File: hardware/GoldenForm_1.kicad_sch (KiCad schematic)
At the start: 37 parts, among them IC1 UVLO, J1 SD_Socket, J2 USB_C_Receptacle_USB2.0_14P, J3 Conn_01x04_Pin, M3 MountingHole x 4, SW1 BOOT, SW2 RESET, U1 Buck_Boost, U2 BNO055, U4 ESP32-S3-WROOM-1

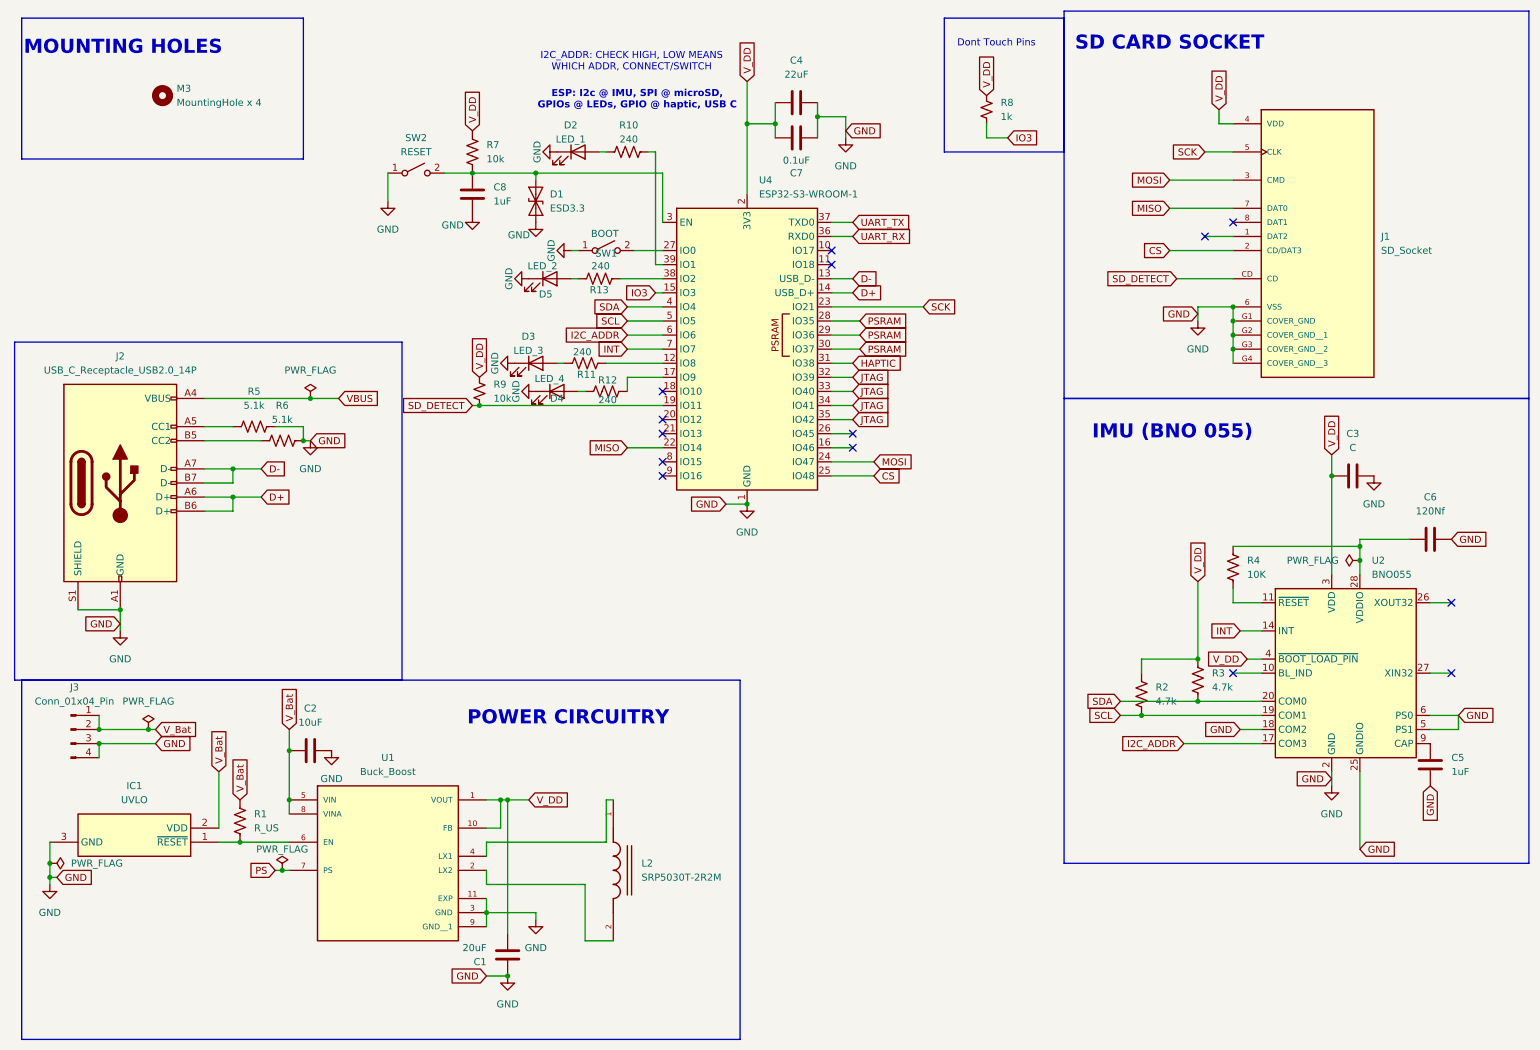
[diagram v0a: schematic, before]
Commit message: some updates to footprints, USBC, buck boost, switch
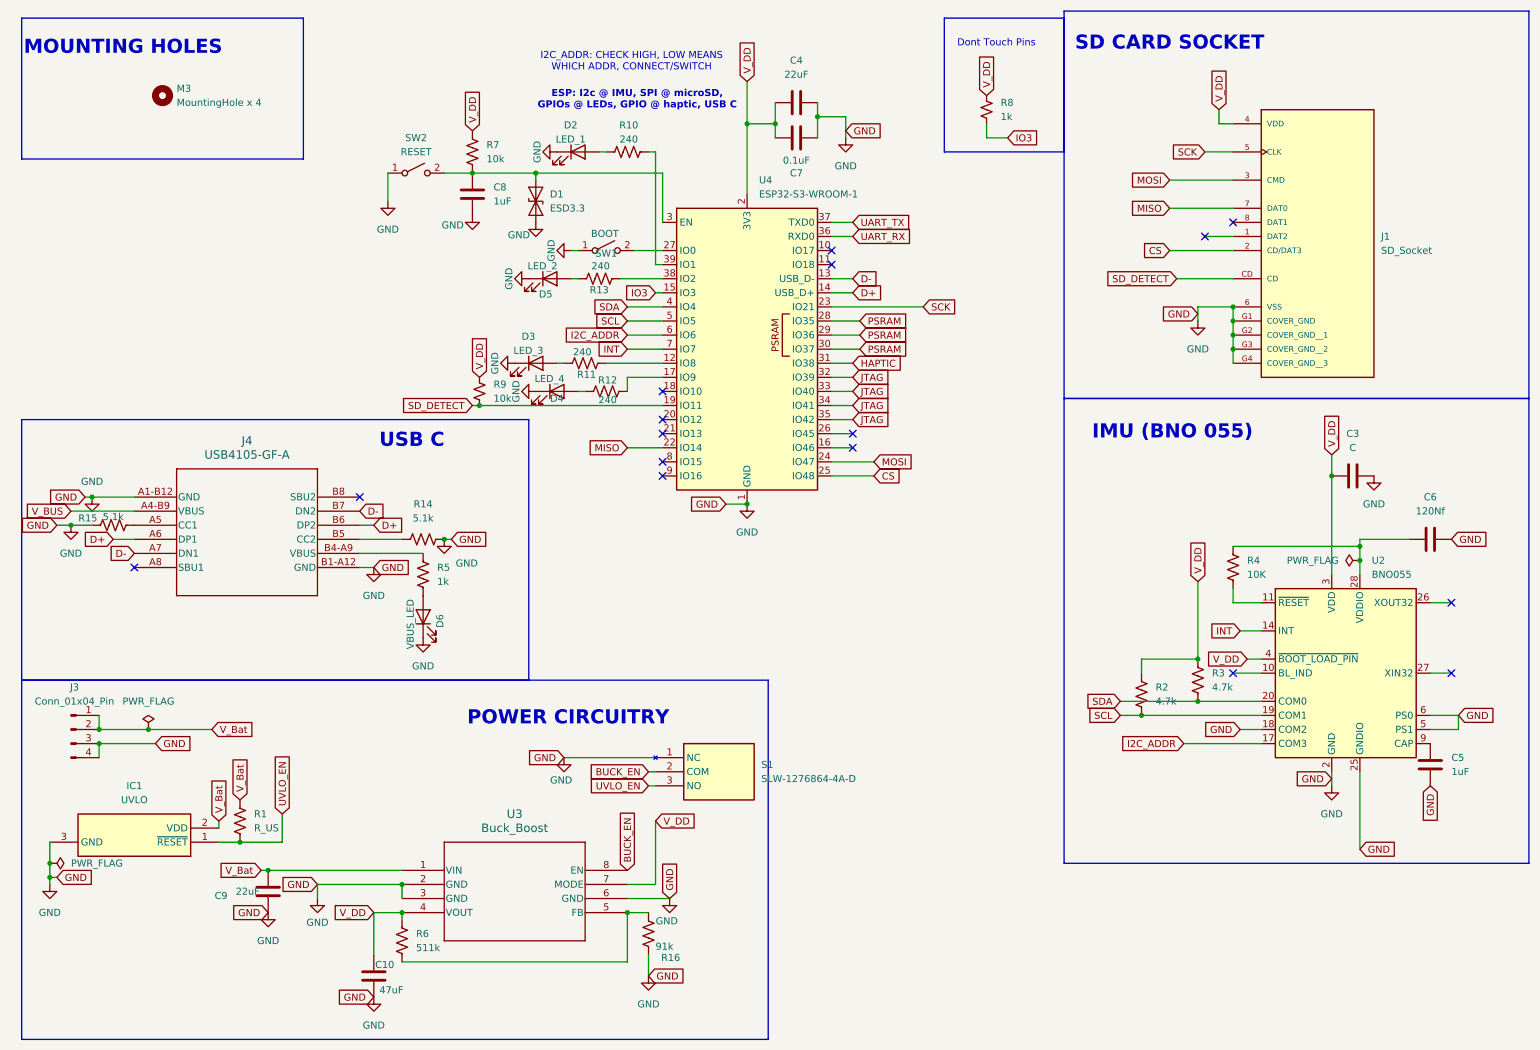
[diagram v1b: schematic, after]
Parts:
- removed C1: 20uF, Capacitor_SMD:C_0805_2012Metric_Pad1.18x1.45mm_HandSolder, symbol Device:C
- removed C2: 10uF, Capacitor_SMD:C_0805_2012Metric_Pad1.18x1.45mm_HandSolder, symbol Device:C
- removed J2: USB_C_Receptacle_USB2.0_14P, Connector_USB:USB_C_Receptacle_GCT_USB4135-GF-A_6P_TopMnt_Horizontal, symbol Connector:USB_C_Receptacle_USB2.0_14P
- removed L2: SRP5030T-2R2M, MyFootprints:INDM5752X300N, symbol MySymbols:SRP5030T-2R2M
- removed U1: Buck_Boost, MyFootprints:SON50P250X250X80-11N, symbol MySymbols:RT6150B-33GQW
- added C10: 47uF, symbol Device:C
- added C9: 22uF, symbol Device:C
- added D6: VBUS_LED, symbol Device:LED
- added J4: USB4105-GF-A, USB4105_GCT, symbol MySymbols:USB4105-GF-A
- added R14, R15: 5.1k, symbol Device:R_US
- added R16: 91k, symbol Device:R_US
- added S1: SLW-1276864-4A-D, SLW12768644AD, symbol MySymbols:SLW-1276864-4A-D
- added U3: Buck_Boost, MICROSIP8_SIU_TEX, symbol MySymbols:TPSM83100SIUR
- R5: value 5.1k -> 1k
- R6: value 5.1k -> 511k
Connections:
- net D+: now also J4.A6 (DP1), J4.B6 (DP2)
- net D-: now also J4.A7 (DN1), J4.B7 (DN2)
- net GND: now also C10.2, C9.2, D6.1 (K), J4.A1-B12 (GND), J4.B1-A12 (GND), R14.2, R15.1, R16.2, S1.1 (NC), U3.2 (GND), U3.3 (GND), U3.6 (GND); no longer R5.2, R6.2
- net V_Bat: now also C9.1, U3.1 (VIN)
- net V_DD: now also R6.1, C10.1, U3.4 (VOUT), U3.7 (MODE)
- net at R5.1: now also D6.2 (A)
- net UVLO_EN: now reaches IC1.1 (~{RESET}), R1.2
- net UVLO_EN: now also S1.3 (NO)
- new net: J4.A5 (CC1), R15.2
- new net: R16.1, R6.2, U3.5 (FB)
- new net: J4.B4-A9 (VBUS), R5.2
- new net: J4.B5 (CC2), R14.1
- new net BUCK_EN: S1.2 (COM), U3.8 (EN)
- new net V_BUS: J4.A4-B9 (VBUS)
- no-connect marks 14 -> 16
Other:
- note added: "USB C"
